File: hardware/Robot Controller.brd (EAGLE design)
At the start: 44.8 x 51.4 mm, 15 parts

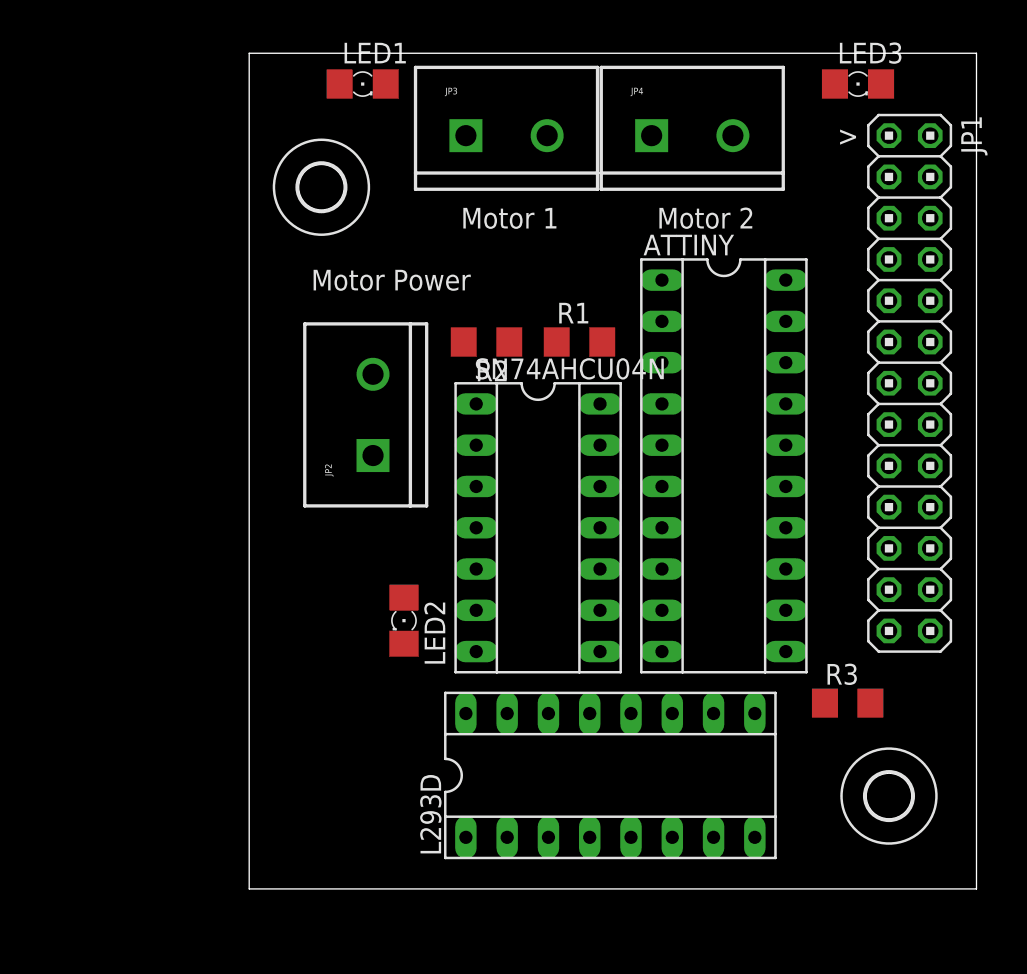
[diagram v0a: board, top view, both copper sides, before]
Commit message: ideas around master/slave robot cores
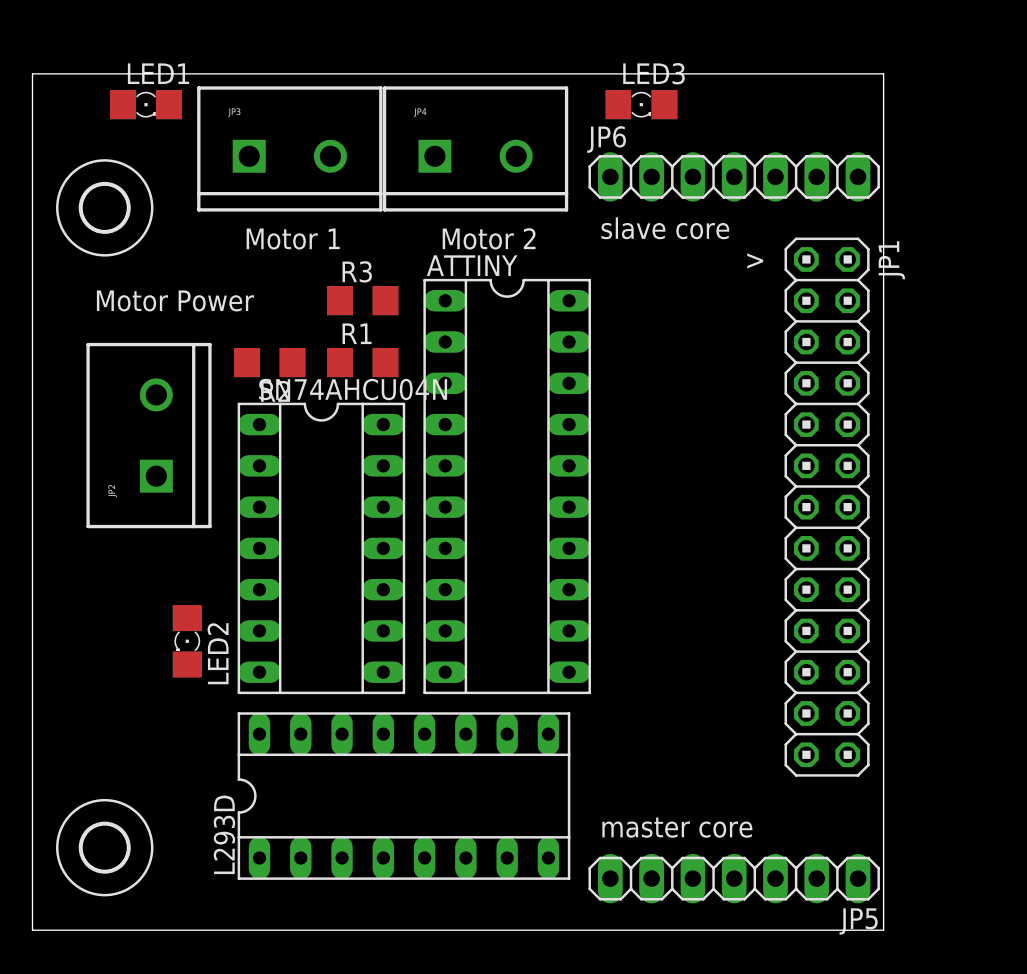
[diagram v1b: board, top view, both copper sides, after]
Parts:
- added JP5, JP6: (no value), pinhead:1X07
- moved H2 48.4 mm to (46.4, 19.7)
- moved R3 38.8 mm to (62.2, 53.3)
- moved JP4 13.4 mm to (66.7, 62.2)
- moved SN74AHCU04N 13.4 mm to (59.7, 38.1)
- moved H1 13.4 mm to (46.4, 59.1)
- moved JP2 13.4 mm to (49.5, 42.5)
- moved JP3 13.4 mm to (55.2, 62.2)
- moved R1 13.4 mm to (62.2, 49.5)
- moved ATTINY 13.4 mm to (71.1, 41.9)
- moved LED2 13.4 mm to (51.4, 32.4)
- moved LED1 13.4 mm to (48.9, 65.4)
- moved LED3 13.4 mm to (79.4, 65.4)
- moved R2 13.4 mm to (56.5, 49.5)
- moved L293D 12.8 mm to (64.8, 22.9)
- moved JP1 9.16 mm to (90.8, 40.6)
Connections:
- net GND: now also JP5.6
- net N$12: now also JP5.1
- net N$4: now also JP5.2
- net N$5: now also JP5.4
- net N$7: now also JP5.3
- net VCC: now also JP5.7
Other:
- board size 44.8 x 51.4 mm -> 52.4 x 52.7 mm
- board text added: "master core"
- board text added: "slave core"

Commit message: WIP dev board
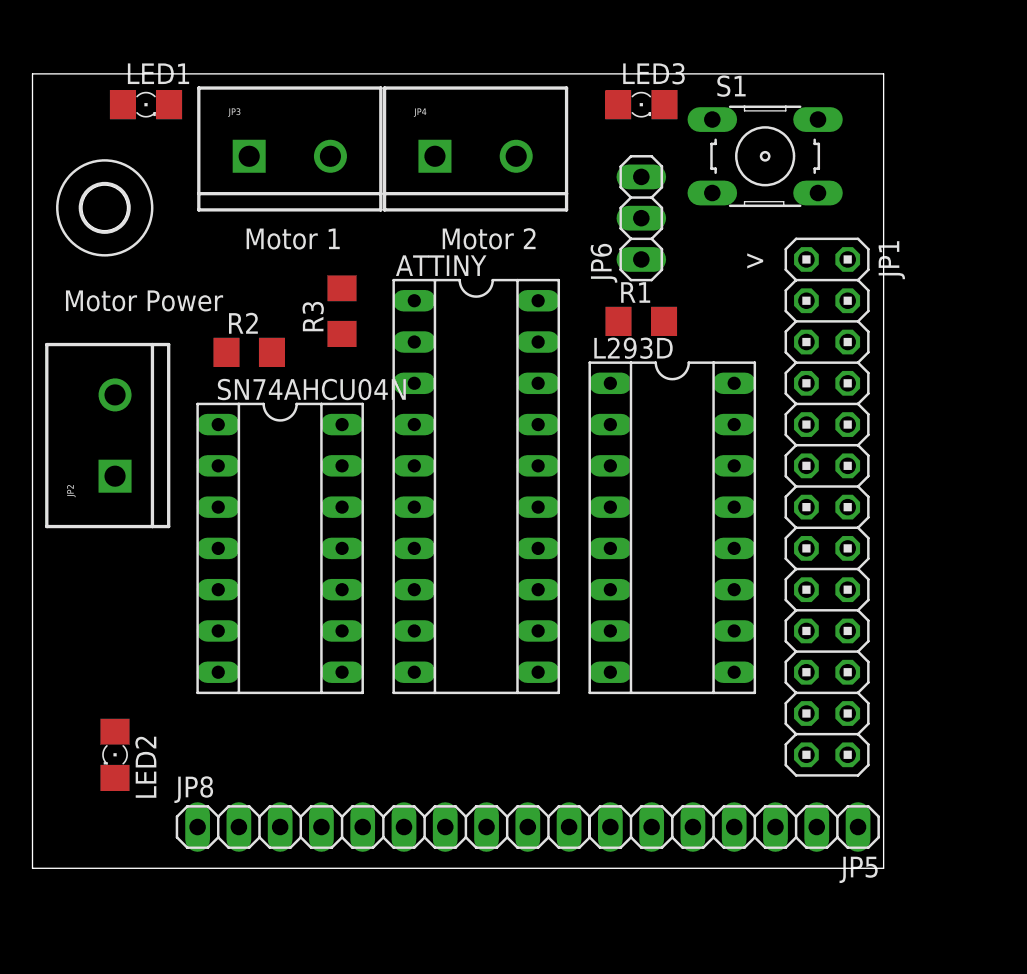
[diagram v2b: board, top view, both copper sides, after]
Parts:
- removed H2: MOUNT-HOLE2.8, holes:2,8
- added JP8: (no value), pinhead:1X10
- added S1: (no value), switch-omron:B3F-10XX
- JP6: device pinhead:1X07 -> pinhead:1X03
- moved L293D 23.3 mm to (81.3, 39.4), turned to 270 degrees
- moved R1 17.3 mm to (79.4, 52.1)
- moved LED2 8.28 mm to (47.0, 25.4)
- moved JP6 6.25 mm to (79.4, 58.4), turned to 90 degrees
- moved JP5 3.17 mm to (85.1, 21.0)
- moved JP2 2.54 mm to (47.0, 42.5)
- moved SN74AHCU04N 2.54 mm to (57.1, 38.1)
- moved ATTINY 1.91 mm to (69.2, 41.9)
- moved R2 1.42 mm to (55.2, 50.2), turned to 0 degrees
- moved R3 1.42 mm to (61.0, 52.7), turned to 90 degrees
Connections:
- new net N$20: ATTINY.5, L293D.10, SN74AHCU04N.11
- new net N$21: JP6.1, R2.1
- new net N$22: L293D.15, SN74AHCU04N.10
- new net N$23: JP6.3, JP8.8
- new net N$24: ATTINY.6, JP8.7
- new net N$25: ATTINY.7, JP8.6
- new net N$26: ATTINY.8, JP8.5
- new net N$27: ATTINY.9, JP8.4
- new net N$28: ATTINY.13, JP8.1
- new net N$29: ATTINY.12, JP8.2
- new net N$30: ATTINY.11, JP8.3
- new net N$31: ATTINY.1, S1.3
- net GND: now also JP8.10, S1.2
- net N$16: now also JP6.2; no longer R2.1
- net VCC: now also JP8.9
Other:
- board size 52.4 x 52.7 mm -> 52.4 x 48.9 mm
- board text removed: "master core"
- board text removed: "slave core"

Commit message: silkscreen work
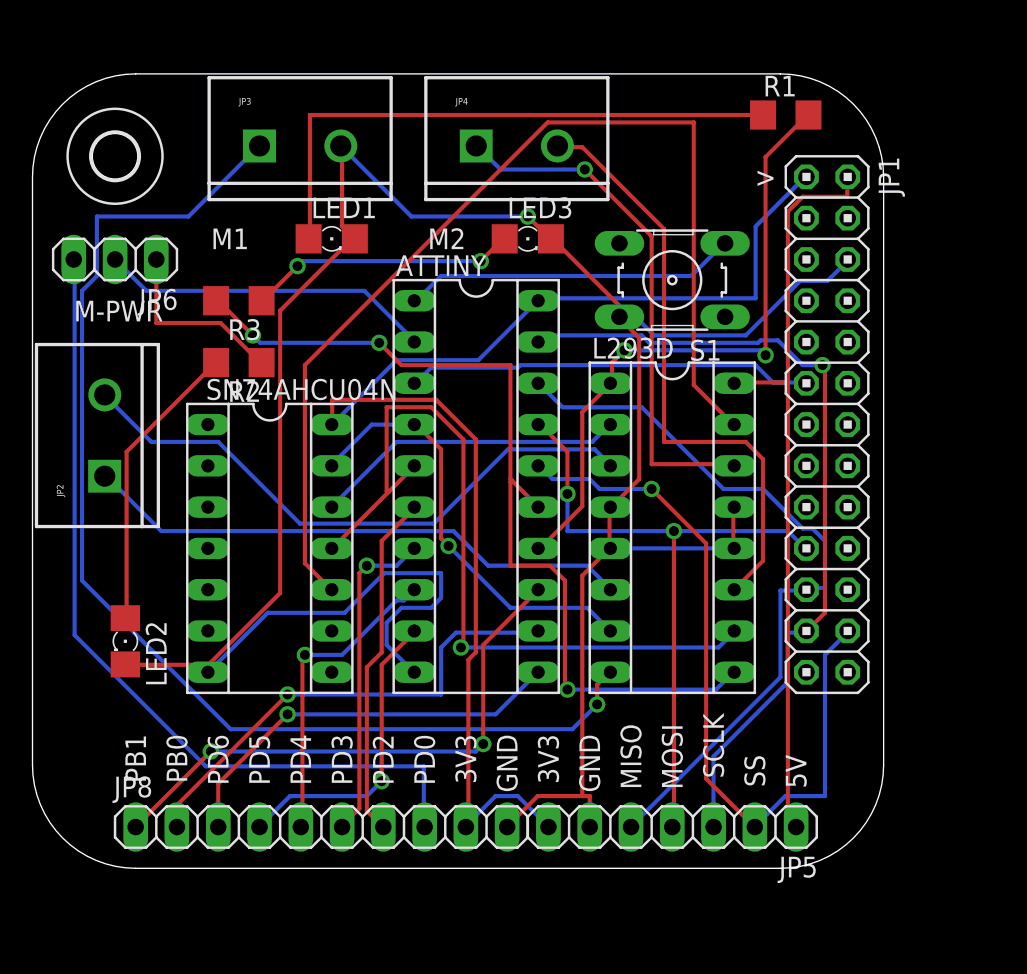
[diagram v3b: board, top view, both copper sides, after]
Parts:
- moved JP6 32.5 mm to (47.0, 55.9), turned to 180 degrees
- moved R1 15.5 mm to (88.3, 64.8)
- moved LED1 14.1 mm to (60.3, 57.1)
- moved LED3 10.8 mm to (72.4, 57.1)
- moved S1 9.53 mm to (81.3, 54.6), turned to 180 degrees
- moved LED2 7.01 mm to (47.6, 32.4)
- moved R3 6.38 mm to (54.6, 53.3), turned to 180 degrees
- moved JP1 5.08 mm to (90.8, 45.7)
- moved JP5 3.81 mm to (81.3, 21.0)
- moved JP8 3.81 mm to (59.7, 21.0)
- moved H1 3.24 mm to (47.0, 62.2)
- moved JP4 2.62 mm to (69.2, 62.9)
- moved JP3 0.90 mm to (55.9, 62.9)
- moved R2 0.90 mm to (54.6, 49.5), turned to 180 degrees
- moved JP2 0.64 mm to (46.4, 42.5)
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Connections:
- net N$6: now also JP5.5
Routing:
- net GND: track 0.00 -> 156.3 mm, vias 0 -> 1
- net VCC: track 0.00 -> 80.3 mm
- net N$10: track 0.00 -> 73.0 mm, vias 0 -> 1
- net N$22: track 0.00 -> 64.3 mm
- net N$11: track 0.00 -> 55.7 mm, vias 0 -> 3
- net N$23: track 0.00 -> 51.7 mm
- net N$7: track 0.00 -> 50.5 mm, vias 0 -> 1
- net N$20: track 0.00 -> 48.2 mm, vias 0 -> 1
- net N$4: track 0.00 -> 46.9 mm, vias 0 -> 1
- net N$12: track 0.00 -> 46.7 mm
- net N$6: track 0.00 -> 45.7 mm
- net N$5: track 0.00 -> 40.8 mm, vias 0 -> 2
- net N$1: track 0.00 -> 39.2 mm, vias 0 -> 2
- net N$19: track 0.00 -> 37.1 mm
- net N$8: track 0.00 -> 36.7 mm
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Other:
- outline, holes or cut-outs redrawn
- board text added: "3V3"
- board text added: "5V"
- board text added: "GND"
- board text added: "M-PWR"
- board text added: "M1"
- board text added: "M2"
- board text added: "MISO"
- board text added: "MOSI"
- board text added: "PB0"
- board text added: "PB1"
- board text added: "PD0"
- board text added: "PD2"
- board text added: "PD3"
- board text added: "PD4"
- board text added: "PD5"
- board text added: "PD6"
- board text added: "SCLK"
- board text added: "SS"
- board text removed: "Motor 1"
- board text removed: "Motor 2"
- board text removed: "Motor Power"
